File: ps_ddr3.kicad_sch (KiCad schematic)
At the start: 79 parts, among them U1 XC7Z010-1CLG400C, U2 H5TC2G83EFR-xxA, U3 H5TC2G83EFR-xxA

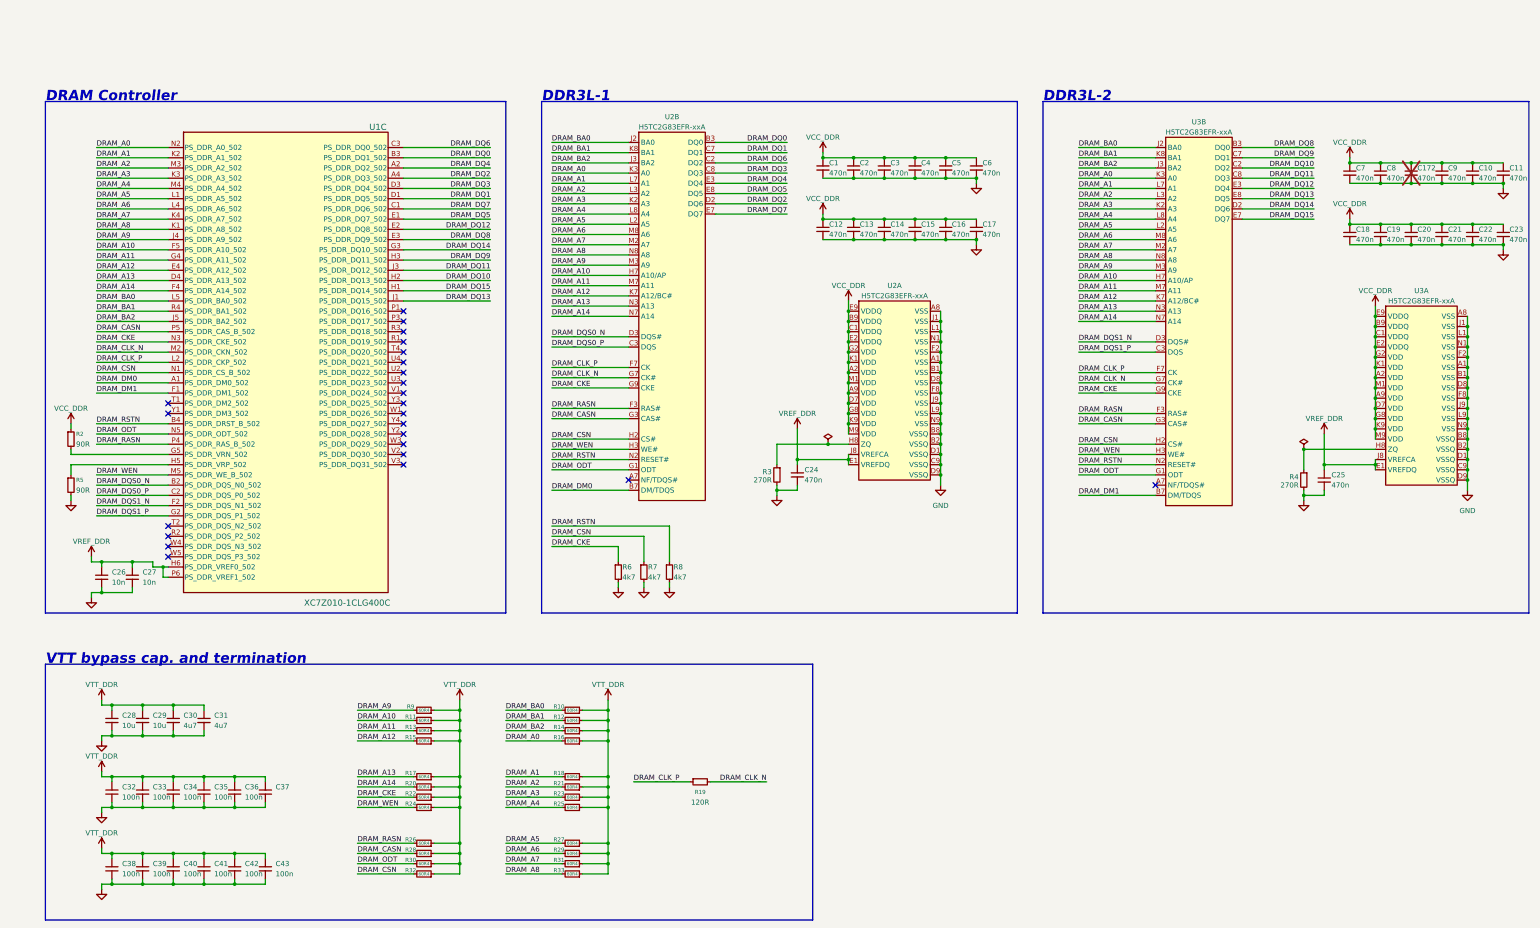
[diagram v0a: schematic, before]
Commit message: add overview
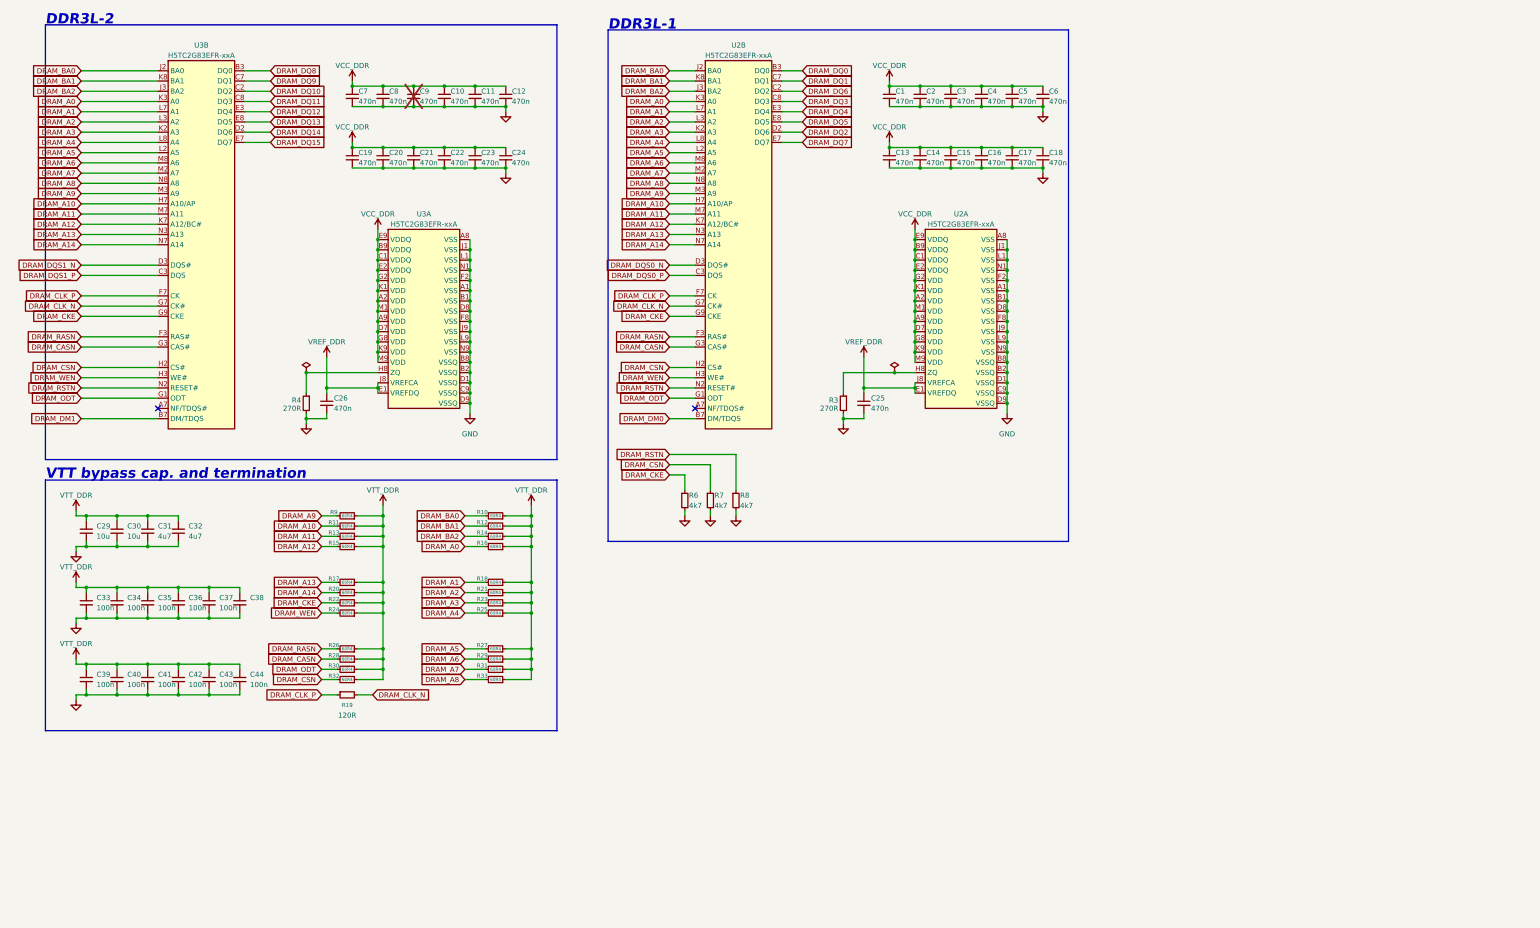
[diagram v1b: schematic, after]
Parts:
- removed C26, C27: 10n, Capacitor_SMD:C_0402_1005Metric, symbol Device:C_Small
- removed R2, R5: 90R, Resistor_SMD:R_0402_1005Metric, symbol Device:R_Small
- removed U1: XC7Z010-1CLG400C, Custom:CLG400_XIL-L, symbol Custom:XC7Z010-1CLG400C
- renumbered C9 to C10, C10 to C11, C11 to C12, C12 to C13, C13 to C14, C14 to C15, C15 to C16, C16 to C17, C17 to C18, C18 to C19, C19 to C20, C20 to C21, C21 to C22, C22 to C23, C23 to C24, C24 to C25, C25 to C26, C28 to C29, C29 to C30, C30 to C31, C31 to C32, C32 to C33, C33 to C34, C34 to C35, C35 to C36, C36 to C37, C37 to C38, C38 to C39, C39 to C40, C40 to C41, C41 to C42, C42 to C43, C43 to C44, C172 to C9
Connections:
- no-connect marks 24 -> 2
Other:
- note removed: "DRAM Controller"
- moved on the sheet: C1, C10, C11, C12, C13, C14, C15, C16, C17, C18, C19, C2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
